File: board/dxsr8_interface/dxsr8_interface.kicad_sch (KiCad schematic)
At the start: 11 parts, among them J1 RJ45, J2 RJ45, J4 NP, K1 Relay_DPDT, K2 Relay_DPDT, U1 ADuM1201AR, U2 ADuM1201AR, U3 AMS1117-5.0

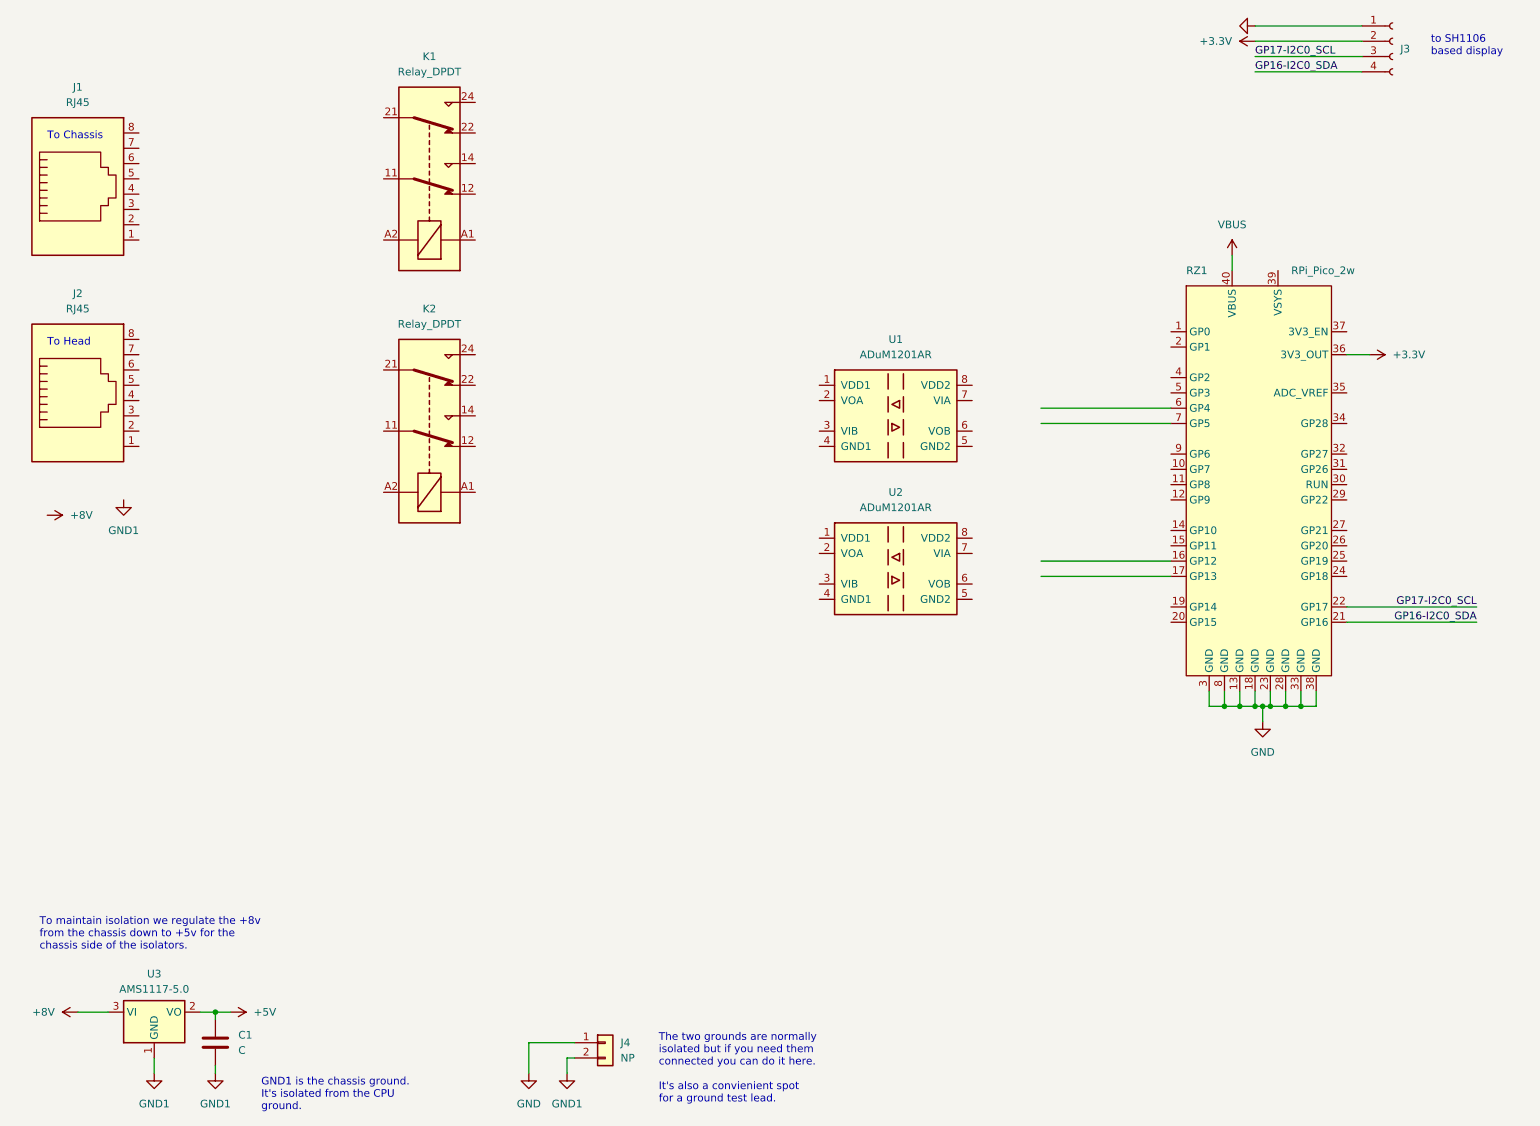
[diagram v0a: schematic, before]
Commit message: work on board design
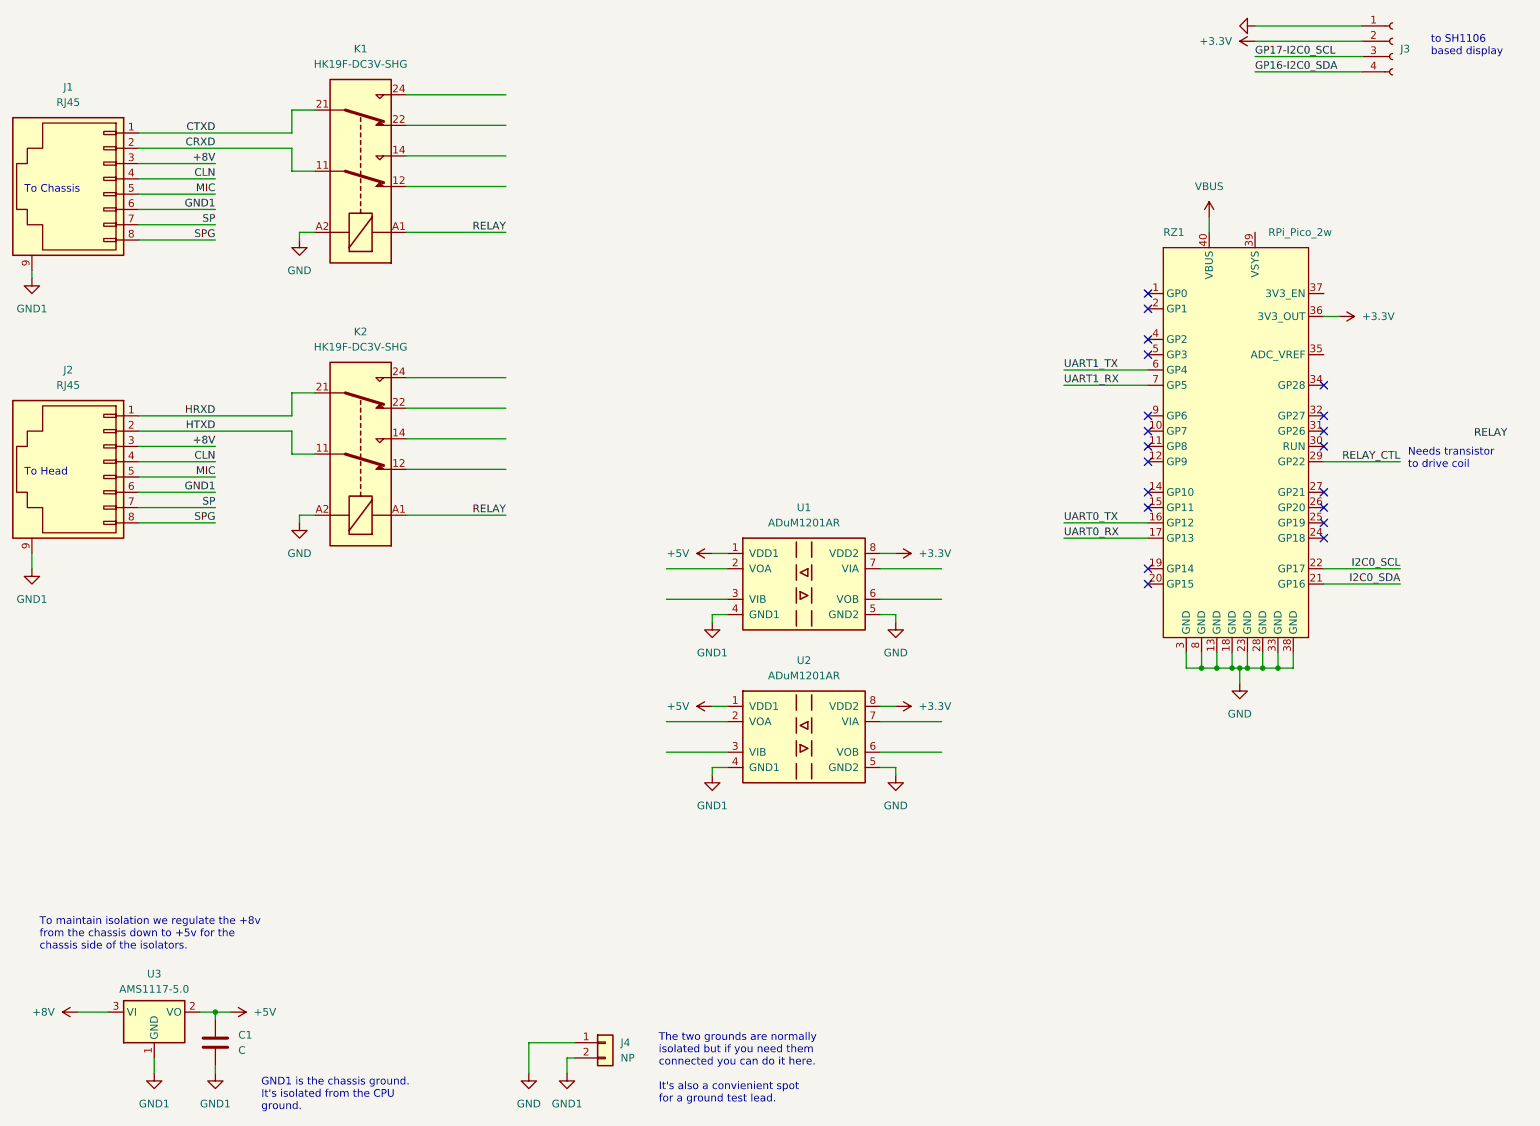
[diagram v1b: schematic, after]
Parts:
- J1, J2: footprint (none) -> digikey-footprints:Ethernet_Jack_ARJC02-111008B; symbol Connector:RJ45 -> dk_Modular-Connectors-Jacks:RJLSE4208101T; Category (none) -> Connectors, Interconnects; DK_Datasheet_Link (none) -> https://cdn.amphenol-icc.com/media/wysiwyg/files/drawing/rj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; DK_Detail_Page (none) -> /product-detail/en/amphenol-icc-commercial-products/RJLSE42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; Digi-Key_PN (none) -> RJLSE4208101TTR-ND; Family (none) -> Modular Connectors - Jacks; MPN (none) -> RJLSE4208101T; Manufacturer (none) -> Amphenol ICC (Commercial Products); Status (none) -> Active
- J3: footprint (none) -> Connector_PinHeader_2.54mm:PinHeader_1x04_P2.54mm_Vertical
- J4: footprint (none) -> Connector_PinHeader_2.54mm:PinHeader_1x02_P2.54mm_Vertical
- K1, K2: value Relay_DPDT -> HK19F-DC3V-SHG; footprint (none) -> Relay_THT:Relay_DPDT_FRT5
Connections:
- net +3.3V: now also U1.8 (VDD2), U2.8 (VDD2)
- net +5V: now also U1.1 (VDD1), U2.1 (VDD1)
- net +8V: now also J1.3, J2.3
- net GND: now also K1.A2, K2.A2, U1.5 (GND2), U2.5 (GND2)
- net GND1: now also J1.6, J1.9, J2.6, J2.9, U1.4 (GND1), U2.4 (GND1)
- net GP16-I2C0_SDA: no longer RZ1.21 (GP16)
- net GP17-I2C0_SCL: no longer RZ1.22 (GP17)
- net UART0_TX: now reaches RZ1.16 (GP12)
- net UART0_RX: now reaches RZ1.17 (GP13)
- net RELAY_CTL: now reaches RZ1.29 (GP22)
- net UART1_TX: now reaches RZ1.6 (GP4)
- net UART1_RX: now reaches RZ1.7 (GP5)
- net CTXD: now reaches J1.1
- net CTXD: now also K1.21
- net CRXD: now reaches J1.2
- net CRXD: now also K1.11
- net CLN: now reaches J1.4
- net CLN: now also J2.4
- net MIC: now reaches J1.5
- net MIC: now also J2.5
- net SP: now reaches J1.7
- net SP: now also J2.7
- net SPG: now reaches J1.8
- net SPG: now also J2.8
- net HRXD: now reaches J2.1
- net HRXD: now also K2.21
- net HTXD: now reaches J2.2
- net HTXD: now also K2.11
- net RELAY: now reaches K1.A1
- net RELAY: now also K2.A1
- new net I2C0_SCL: RZ1.22 (GP17)
- new net I2C0_SDA: RZ1.21 (GP16)
- no-connect marks 0 -> 20
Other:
- note added: "Needs transistor to drive coil"
- moved on the sheet: K1, K2, RZ1, U1, U2
